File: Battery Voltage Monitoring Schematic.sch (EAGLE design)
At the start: 13 parts, among them U1 INA3221.

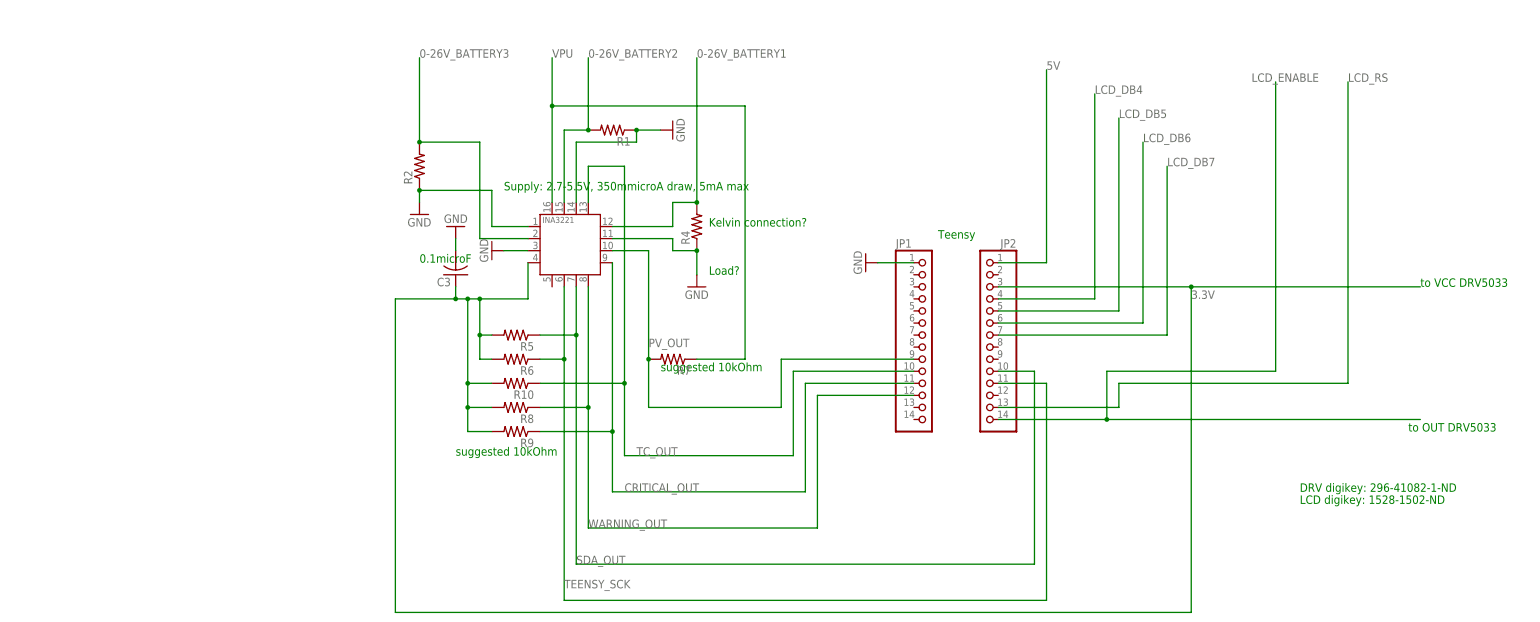
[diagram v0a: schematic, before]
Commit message: Add files via upload
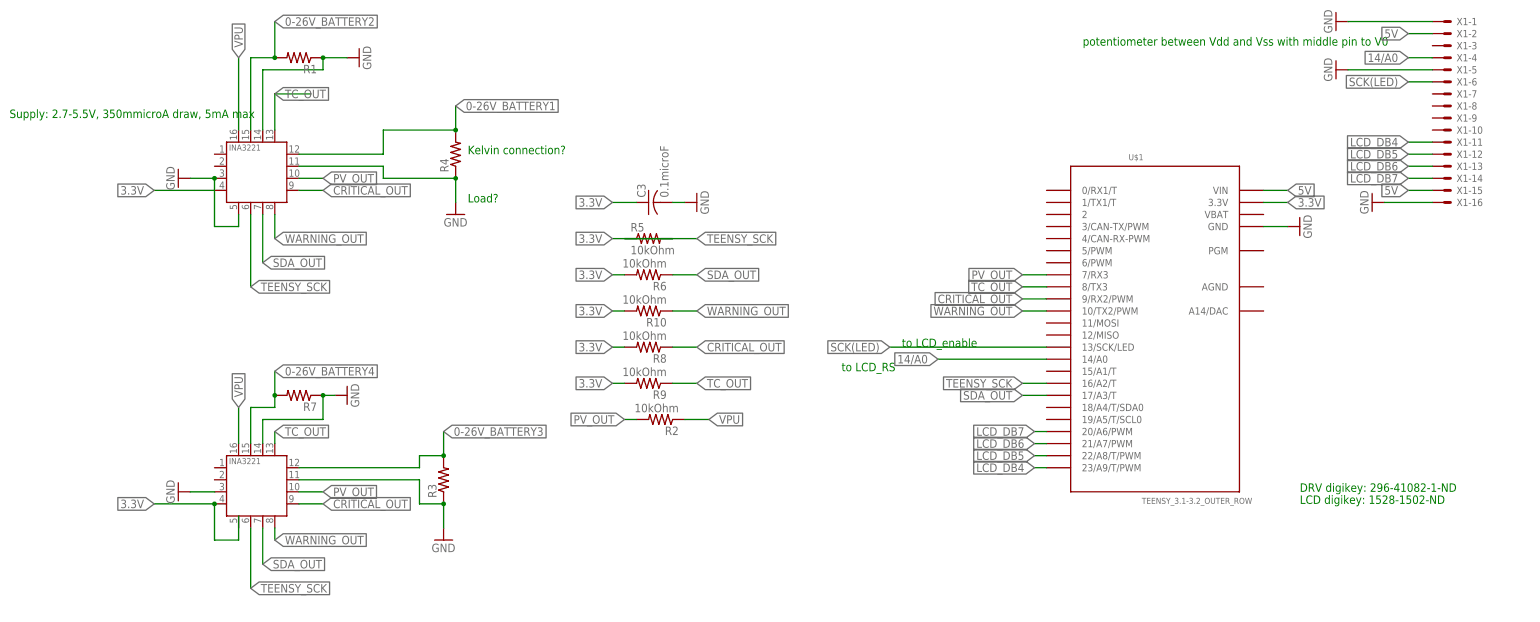
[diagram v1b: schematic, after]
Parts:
- removed JP1, JP2: (no value), pinhead:PINHD-1X14
- added R3: (no value), rcl:R-US_R0805
- added U$1: TEENSY_3.1-3.2_OUTER_ROW, Teensy_3_and_LC_Series_Boards_v1.4:TEENSY_3.1-3.2_OUTER_ROW
- added U2: INA3221., INA3221:INA3221.
- added X1: (no value), con-molex:KK-156-16
- C3: value (none) -> 0.1microF
- R10, R2, R5, R6, R8, R9: value (none) -> 10kOhm
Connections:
- removed net LCD_ENABLE: JP2.14
- removed net LCD_RS: JP2.13
- new net 0-26V_BATTERY4: R7.2, U2.IN+2
- new net 14/A0: U$1.14/A0, X1-4.S
- new net LCD_DB4: U$1.23/A9/T/PWM, X1-11.S
- new net SCK(LED): U$1.13/SCK/LED, X1-6.S
- net 0-26V_BATTERY3: now also R3.2, U2.IN+1; no longer R2.2, U1.IN+3
- net 3.3V: now also U$1.3.3V, U2.VS; no longer JP2.3
- net 5V: now also U$1.VIN, X1-15.S, X1-2.S; no longer JP2.1
- net CRITICAL_OUT: now also R8.1, U$1.9/RX2/PWM, U2.CRITICAL; no longer JP1.11, R9.1
- net GND: now also R3.1, R7.1, U$1.GND, U1.A0, U2.GND, U2.IN-1, U2.IN-2, X1-1.S, X1-16.S, X1-5.S; no longer JP1.1, R2.1, U1.IN-3
- net LCD_DB5: now also U$1.22/A8/T/PWM, X1-12.S; no longer JP2.5
- net LCD_DB6: now also U$1.21/A7/PWM, X1-13.S; no longer JP2.6
- net LCD_DB7: now also U$1.20/A6/PWM, X1-14.S; no longer JP2.7
- net PV_OUT: now also R2.2, U$1.7/RX3, U2.PV; no longer JP1.9, R7.2
- net SDA_OUT: now also R6.1, U$1.17/A3/T, U2.SDA; no longer JP2.10, R5.1
- net TC_OUT: now also R9.1, U$1.8/TX3, U2.TC; no longer JP1.10, R10.1
- net TEENSY_SCK: now also R5.1, U$1.16/A2/T, U2.SCL; no longer JP2.11, R6.1
- net VPU: now also R2.1, U2.VPU; no longer R7.1
- net WARNING_OUT: now also R10.1, U$1.10/TX2/PWM, U2.WARNING; no longer JP1.12, R8.1
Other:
- note added: "potentiometer between Vdd and Vss with middle pin to V0"
- note added: "to LCD_RS"
- note added: "to LCD_enable"
- note removed: "0.1microF"
- note removed: "Teensy"
- note removed: "suggested 10kOhm"
- note removed: "to OUT DRV5033"
- note removed: "to VCC DRV5033"
- moved on the sheet: C3, R1, R10, R2, R4, R5, R6, R7, R8, R9
